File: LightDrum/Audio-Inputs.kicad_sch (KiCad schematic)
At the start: 18 parts, among them J4 XLR3, J5 SJ-43515RS-SMT-TR, K3 2-SW-RELAY, U41 SSM3K361R_SOT23F, U7 OPA1652

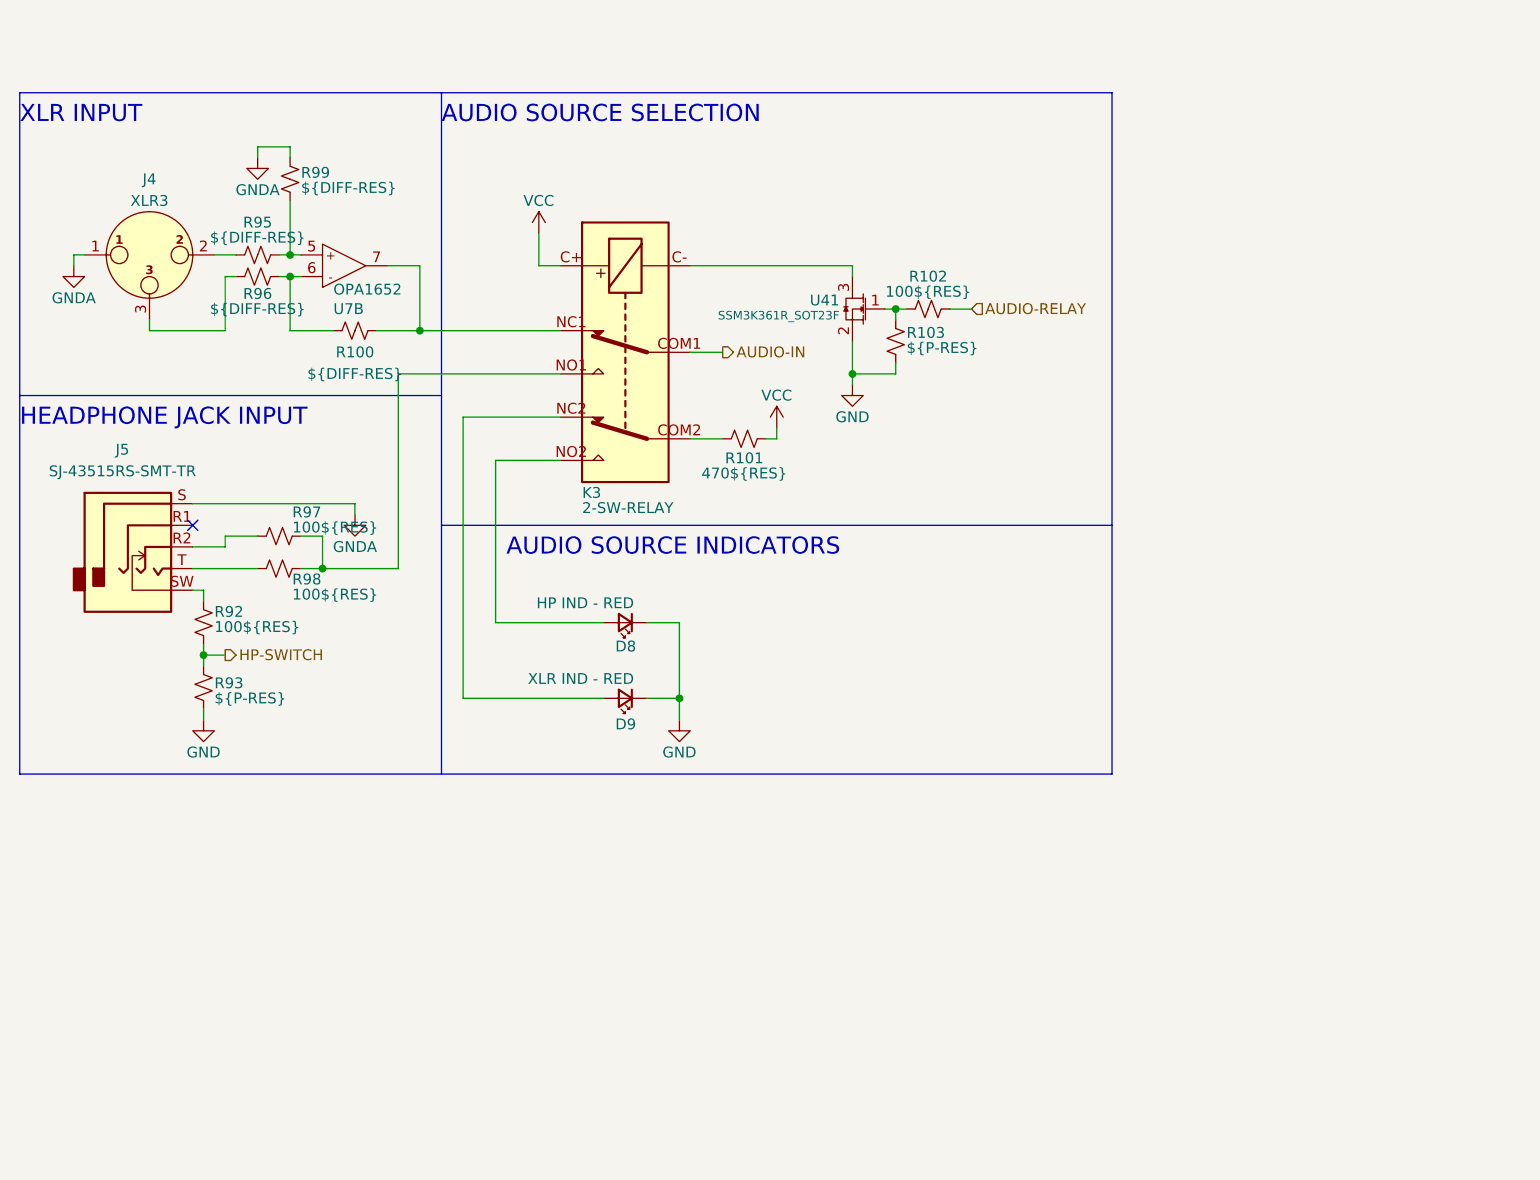
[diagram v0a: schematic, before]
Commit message: First pass over schematic (WIP)
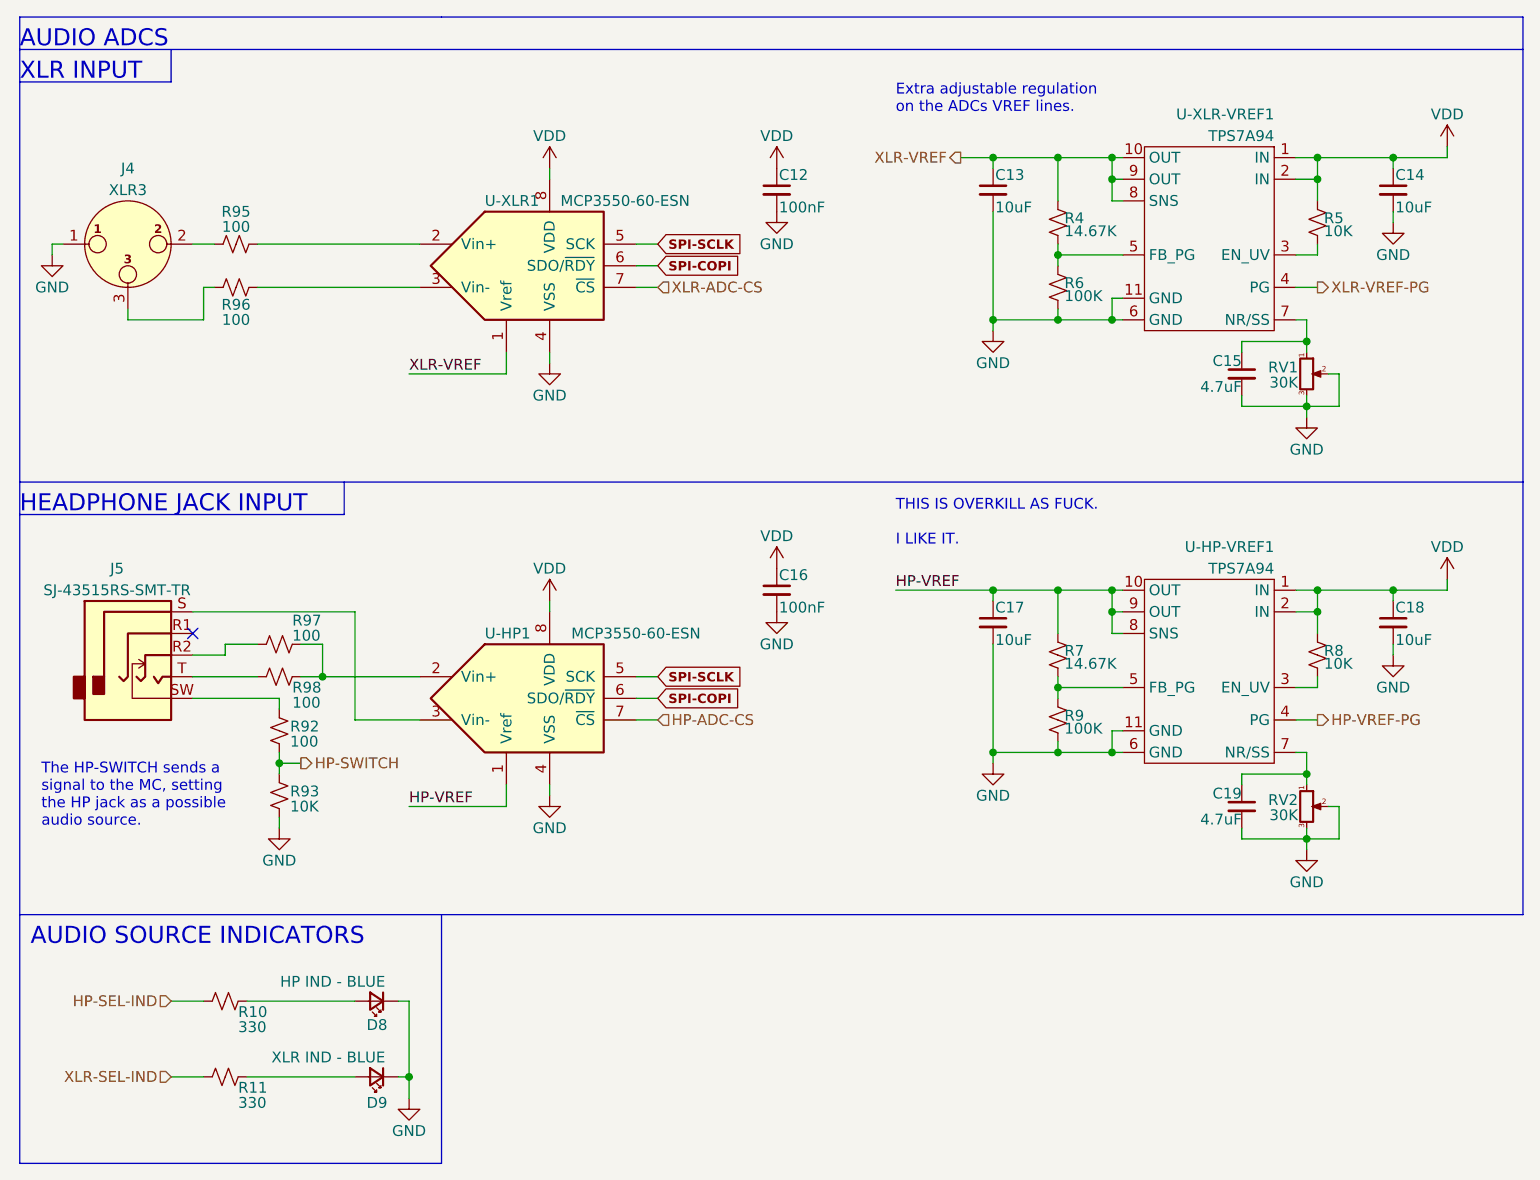
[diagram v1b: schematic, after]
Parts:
- removed K3: 2-SW-RELAY, Daxxn_Relays:AGQ200S4HZ, symbol Daxxn_Relays:2-SW-RELAY
- removed R100, R99: ${DIFF-RES}, Resistor_SMD:R_0805_2012Metric, symbol Device:R_Small_US
- removed R101: 470${RES}, Resistor_SMD:R_0805_2012Metric, symbol Device:R_Small_US
- removed R102: 100${RES}, Resistor_SMD:R_0805_2012Metric, symbol Device:R_Small_US
- removed R103: ${P-RES}, Resistor_SMD:R_0805_2012Metric, symbol Device:R_Small_US
- removed U41: SSM3K361R_SOT23F, Package_TO_SOT_SMD:SOT-23, symbol Daxxn_Transistors:SSM3K361R_SOT23F
- removed U7: OPA1652, Package_SO:VSSOP-8_3.0x3.0mm_P0.65mm, symbol Daxxn_OPAMP:OPA1652
- added C12, C16: 100nF, Capacitor_SMD:C_0603_1608Metric, symbol Device:C_Small
- added C13, C14, C17, C18: 10uF, Capacitor_SMD:C_1210_3225Metric, symbol Device:C_Small
- added C15, C19: 4.7uF, Capacitor_SMD:C_0805_2012Metric, symbol Device:C_Small
- added R10, R11: 330, Resistor_SMD:R_0805_2012Metric, symbol Device:R_Small_US
- added R4, R7: 14.67K, Resistor_SMD:R_0603_1608Metric, symbol Device:R_Small_US
- added R5, R8: 10K, Resistor_SMD:R_0603_1608Metric, symbol Device:R_Small_US
- added R6, R9: 100K, Resistor_SMD:R_0603_1608Metric, symbol Device:R_Small_US
- added RV1, RV2: 30K, Potentiometer_SMD:Potentiometer_Bourns_TC33X_Vertical, symbol Device:R_Potentiometer_Small
- added U-HP-VREF1, U-XLR-VREF1: TPS7A94, Daxxn_Packages:WSON-10-1EP_3x3mm, symbol Daxxn_Regulators:TPS7A94
- added U-HP1, U-XLR1: MCP3550-60-ESN, symbol Analog_ADC:MCP3550-60-ESN
- D8: value HP IND - RED -> HP IND - BLUE
- D9: value XLR IND - RED -> XLR IND - BLUE
- R92, R97, R98: value 100${RES} -> 100
- R93: value ${P-RES} -> 10K
- R95, R96: value ${DIFF-RES} -> 100
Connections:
- net GND: now also J4.1, C12.2, C13.2, C14.2, C15.2, C16.2, C17.2, C18.2, C19.2, R6.2, R9.2, RV1.2, RV1.3, RV2.2, RV2.3, U-HP-VREF1.11 (GND), U-HP-VREF1.6 (GND), U-HP1.4 (VSS), U-XLR-VREF1.11 (GND), U-XLR-VREF1.6 (GND), U-XLR1.4 (VSS)
- net at R97.2, R98.2: now also U-HP1.2 (Vin+)
- net at R96.2: now also U-XLR1.3 (Vin-)
- net at R95.2: now also U-XLR1.2 (Vin+)
- net at D9.2 (A): now also R11.2
- net at D8.2 (A): now also R10.2
- net GNDA: no longer names the net of J5.S
- net GNDA: now also U-HP1.3 (Vin-); no longer J4.1
- new net: R5.2, U-XLR-VREF1.3 (EN_UV)
- new net: R4.2, R6.1, U-XLR-VREF1.5 (FB_PG)
- new net: C15.1, RV1.1, U-XLR-VREF1.7 (NR/SS)
- new net: R7.2, R9.1, U-HP-VREF1.5 (FB_PG)
- new net: R8.2, U-HP-VREF1.3 (EN_UV)
- new net: C19.1, RV2.1, U-HP-VREF1.7 (NR/SS)
- new net HP-ADC-CS: U-HP1.7 (~{CS})
- new net HP-SEL-IND: R10.1
- new net HP-VREF: C17.1, R7.1, U-HP-VREF1.10 (OUT), U-HP-VREF1.8 (SNS), U-HP-VREF1.9 (OUT), U-HP1.1 (Vref)
- new net HP-VREF-PG: U-HP-VREF1.4 (PG)
- new net SPI-COPI: U-HP1.6 (SDO/~{RDY}), U-XLR1.6 (SDO/~{RDY})
- new net SPI-SCLK: U-HP1.5 (SCK), U-XLR1.5 (SCK)
- new net VDD: C12.1, C14.1, C16.1, C18.1, R5.1, R8.1, U-HP-VREF1.1 (IN), U-HP-VREF1.2 (IN), U-HP1.8 (VDD), U-XLR-VREF1.1 (IN), U-XLR-VREF1.2 (IN), U-XLR1.8 (VDD)
- new net XLR-ADC-CS: U-XLR1.7 (~{CS})
- new net XLR-SEL-IND: R11.1
- new net XLR-VREF: C13.1, R4.1, U-XLR-VREF1.10 (OUT), U-XLR-VREF1.8 (SNS), U-XLR-VREF1.9 (OUT), U-XLR1.1 (Vref)
- new net XLR-VREF-PG: U-XLR-VREF1.4 (PG)
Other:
- note added: "AUDIO ADCS"
- note added: "Extra adjustable regulation on the ADCs VREF lines."
- note added: "THIS IS OVERKILL AS FUCK. I LIKE IT."
- note added: "The HP-SWITCH sends a signal to the MC, setting the HP jack as a possible audio source."
- note removed: "AUDIO SOURCE SELECTION"
- moved on the sheet: D8, D9, J4, J5, R92, R93, R95, R96, R97, R98
